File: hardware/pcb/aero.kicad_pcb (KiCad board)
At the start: 4 copper layers, 84 parts, among them CON1 USB-MICRO-B, CON2 MMCX_CONN, J1 CORTEX_DBG_CONN, J2 LiPoly_Conn, Q1 BSS138, SW1 SW_PUSH, U1 STM32L151C8, U10 BU4SU69G2, U11 BU4SU69G2, U12 NC7WZ17, U13 u-blox_max-7c/q, U14 MAX2659, U2 nRF8001, U3 2450BM14A0002, U4 ms5611, U5 BMX055, U6 AT45DB321E, U7 BQ24040DSQ, U8 TPS783, U9 TPS61041, Y1 Crystal, Y2 32.768KHz, Y3 16MHz

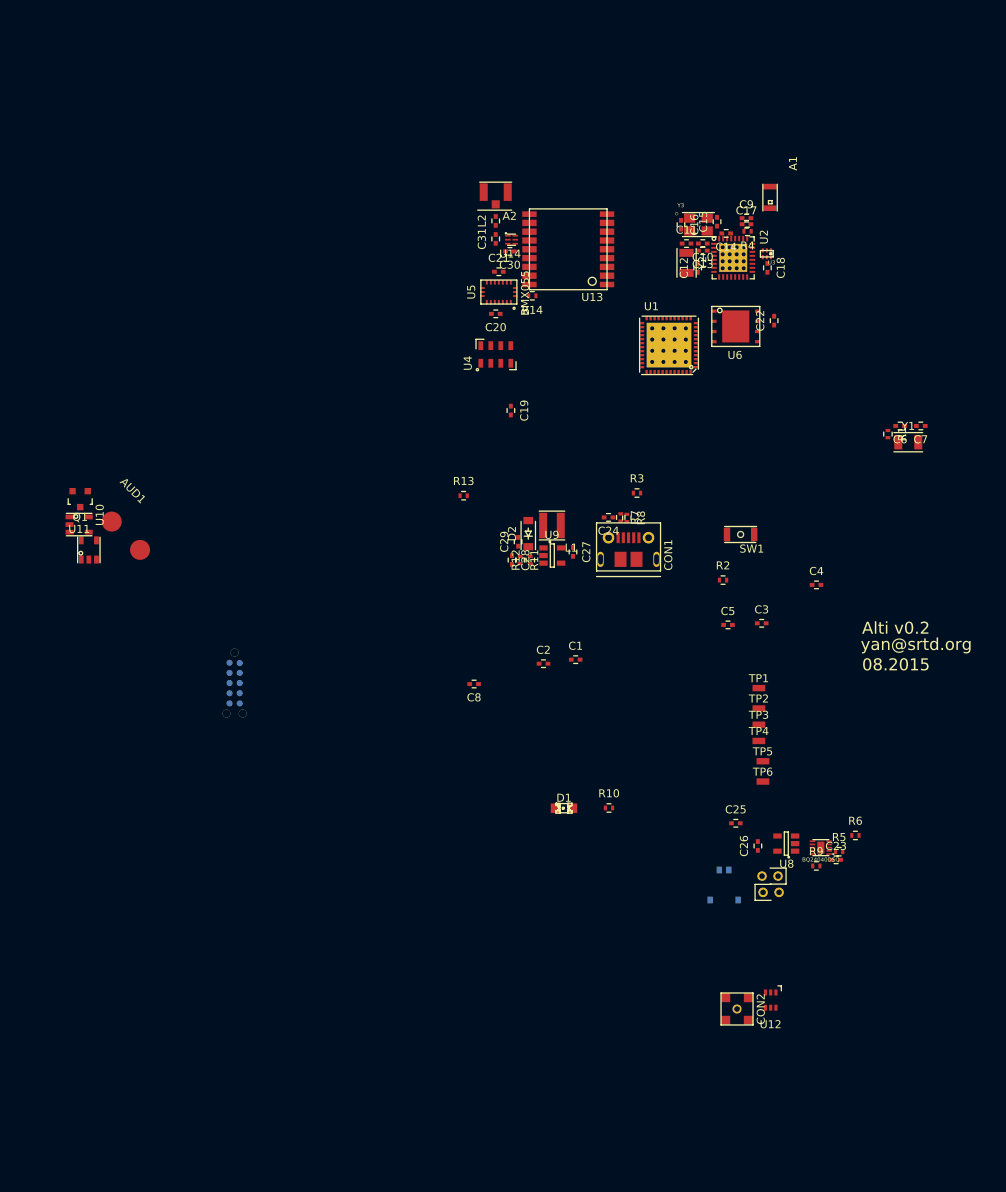
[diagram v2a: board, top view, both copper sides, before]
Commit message: ver2 is nearing completion.
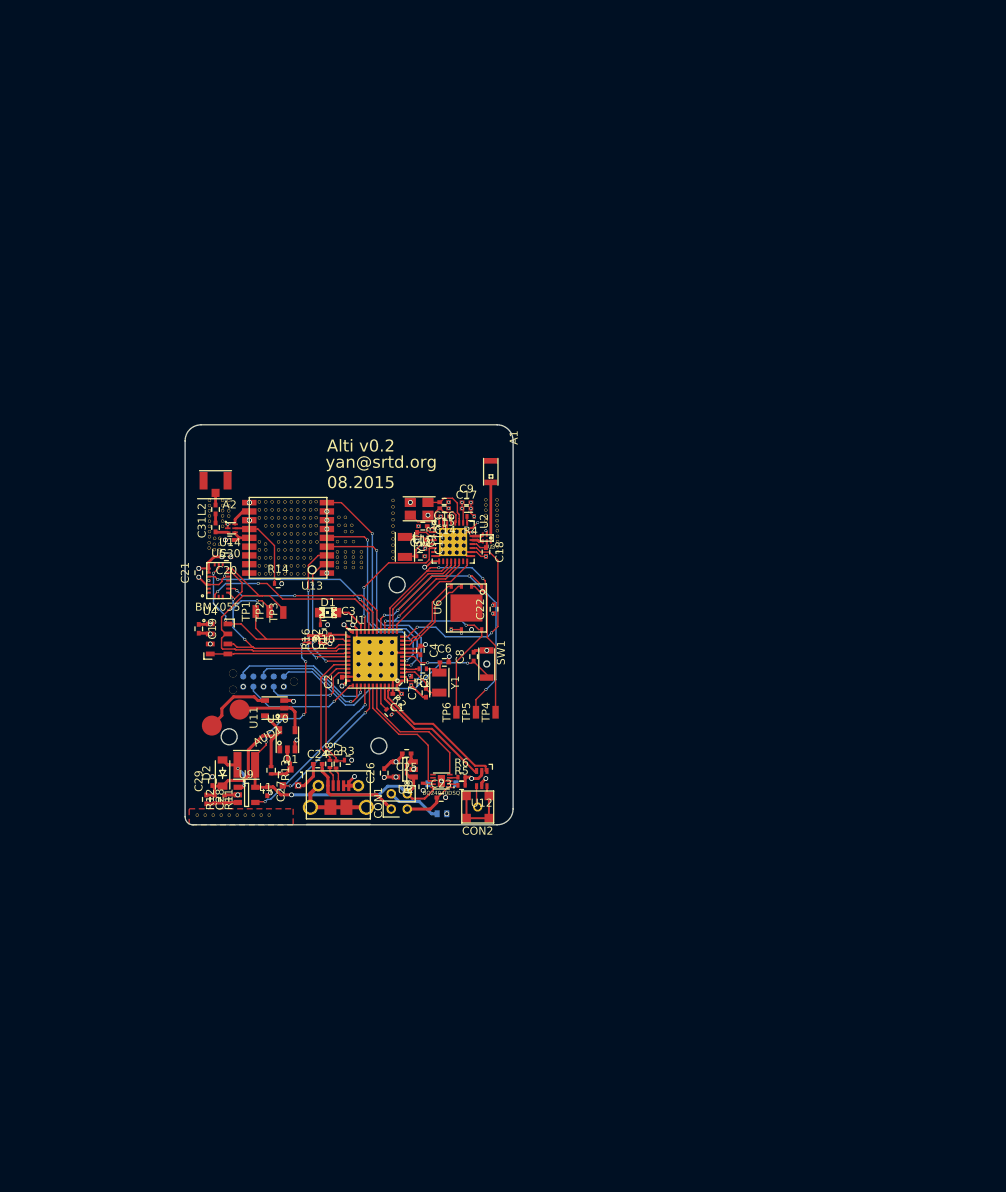
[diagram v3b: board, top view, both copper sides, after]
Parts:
- removed REF**: v, aero:Via_Stitch
- added C32: 100nF, Capacitors_SMD:C_0402, F.Cu at (143.1, 91.8)
- added R15: 10m, Resistors_SMD:R_0402, F.Cu at (140.5, 91.8)
- added R16: 10m, Resistors_SMD:R_0402, F.Cu at (141.9, 91.8)
- added REF**11101: v, aero:Via_Stitch, F.Cu at (141.4, 74.6)
- added REF**11102: v, aero:Via_Stitch, F.Cu at (141.4, 75.6)
- added REF**11103: v, aero:Via_Stitch, F.Cu at (141.4, 76.6)
- added REF**11104: v, aero:Via_Stitch, F.Cu at (141.4, 77.6)
- added REF**11105: v, aero:Via_Stitch, F.Cu at (141.4, 78.6)
- added REF**11106: v, aero:Via_Stitch, F.Cu at (141.5, 79.6)
- added REF**1111: v, aero:Via_Stitch, F.Cu at (134.3, 74.6)
- added REF**11110: v, aero:Via_Stitch, F.Cu at (134.3, 83.6)
- added REF**111101: v, aero:Via_Stitch, F.Cu at (135.5, 113.8)
- added REF**11111: v, aero:Via_Stitch, F.Cu at (126.5, 113.8)
- added REF**11111111: v, aero:Via_Stitch, F.Cu at (128.0, 80.4)
- added REF**11111111: v, aero:Via_Stitch, F.Cu at (128.0, 79.7)
- added REF**11111111: v, aero:Via_Stitch, F.Cu at (128.0, 79.0)
- added REF**11111112: v, aero:Via_Stitch, F.Cu at (129.3, 80.6)
- added REF**11111112: v, aero:Via_Stitch, F.Cu at (129.3, 79.9)
- added REF**11111112: v, aero:Via_Stitch, F.Cu at (129.3, 79.2)
- added REF**11111112: v, aero:Via_Stitch, F.Cu at (128.0, 78.3)
- added REF**11111113: v, aero:Via_Stitch, F.Cu at (128.7, 80.6)
- added REF**11111113: v, aero:Via_Stitch, F.Cu at (128.7, 79.9)
- added REF**11111113: v, aero:Via_Stitch, F.Cu at (128.7, 79.2)
- added REF**11111113: v, aero:Via_Stitch, F.Cu at (129.7, 77.7)
- added REF**11111113: v, aero:Via_Stitch, F.Cu at (128.0, 77.7)
- added REF**11111114: v, aero:Via_Stitch, F.Cu at (129.7, 77.0)
- added REF**11111114: v, aero:Via_Stitch, F.Cu at (128.0, 77.0)
- added REF**11111115: v, aero:Via_Stitch, F.Cu at (130.4, 76.4)
- added REF**11111115: v, aero:Via_Stitch, F.Cu at (129.7, 76.4)
- added REF**11111115: v, aero:Via_Stitch, F.Cu at (128.0, 76.4)
- added REF**11111116: v, aero:Via_Stitch, F.Cu at (130.4, 75.8)
- added REF**11111116: v, aero:Via_Stitch, F.Cu at (129.7, 75.7)
- added REF**11111116: v, aero:Via_Stitch, F.Cu at (128.0, 75.7)
- added REF**11111117: v, aero:Via_Stitch, F.Cu at (130.4, 75.1)
- added REF**11111117: v, aero:Via_Stitch, F.Cu at (129.7, 75.1)
- added REF**11111117: v, aero:Via_Stitch, F.Cu at (128.0, 75.1)
- added REF**11111118: v, aero:Via_Stitch, F.Cu at (130.4, 74.5)
- added REF**11111118: v, aero:Via_Stitch, F.Cu at (129.7, 74.4)
- added REF**11111118: v, aero:Via_Stitch, F.Cu at (128.0, 74.4)
- added REF**1112: v, aero:Via_Stitch, F.Cu at (134.3, 75.6)
- added REF**11121: v, aero:Via_Stitch, F.Cu at (127.5, 113.8)
- added REF**1113: v, aero:Via_Stitch, F.Cu at (134.3, 76.6)
- added REF**11131: v, aero:Via_Stitch, F.Cu at (128.5, 113.8)
- added REF**11141: v, aero:Via_Stitch, F.Cu at (129.5, 113.8)
- added REF**11151: v, aero:Via_Stitch, F.Cu at (130.5, 113.8)
- added REF**1116: v, aero:Via_Stitch, F.Cu at (134.3, 79.6)
- added REF**11161: v, aero:Via_Stitch, F.Cu at (131.5, 113.8)
- added REF**1117: v, aero:Via_Stitch, F.Cu at (134.3, 80.6)
- added REF**11171: v, aero:Via_Stitch, F.Cu at (132.5, 113.8)
- added REF**1118: v, aero:Via_Stitch, F.Cu at (134.3, 81.6)
- added REF**11181: v, aero:Via_Stitch, F.Cu at (133.5, 113.8)
- added REF**1119: v, aero:Via_Stitch, F.Cu at (134.3, 82.6)
- added REF**11191: v, aero:Via_Stitch, F.Cu at (134.5, 113.8)
- added REF**1121: v, aero:Via_Stitch, F.Cu at (135.1, 74.6)
- added REF**11210: v, aero:Via_Stitch, F.Cu at (135.1, 83.6)
- added REF**1122: v, aero:Via_Stitch, F.Cu at (135.1, 75.6)
- added REF**1123: v, aero:Via_Stitch, F.Cu at (135.1, 76.6)
- added REF**1124: v, aero:Via_Stitch, F.Cu at (135.1, 77.6)
- added REF**1126: v, aero:Via_Stitch, F.Cu at (135.1, 79.9)
- added REF**1127: v, aero:Via_Stitch, F.Cu at (135.1, 80.6)
- added REF**1128: v, aero:Via_Stitch, F.Cu at (135.1, 81.6)
- added REF**1129: v, aero:Via_Stitch, F.Cu at (135.1, 82.6)
- added REF**1131: v, aero:Via_Stitch, F.Cu at (135.9, 74.6)
- added REF**11310: v, aero:Via_Stitch, F.Cu at (135.7, 83.6)
- added REF**1132: v, aero:Via_Stitch, F.Cu at (135.9, 75.6)
- added REF**1133: v, aero:Via_Stitch, F.Cu at (135.9, 76.6)
- added REF**1134: v, aero:Via_Stitch, F.Cu at (135.9, 77.6)
- added REF**1135: v, aero:Via_Stitch, F.Cu at (135.9, 78.6)
- added REF**1138: v, aero:Via_Stitch, F.Cu at (135.7, 81.6)
- added REF**1139: v, aero:Via_Stitch, F.Cu at (135.7, 82.6)
- added REF**1141: v, aero:Via_Stitch, F.Cu at (136.7, 74.6)
- added REF**11410: v, aero:Via_Stitch, F.Cu at (136.7, 83.6)
- added REF**1142: v, aero:Via_Stitch, F.Cu at (136.7, 75.6)
- added REF**1143: v, aero:Via_Stitch, F.Cu at (136.7, 76.6)
- added REF**1144: v, aero:Via_Stitch, F.Cu at (136.7, 77.6)
- added REF**1145: v, aero:Via_Stitch, F.Cu at (136.7, 78.6)
- added REF**1146: v, aero:Via_Stitch, F.Cu at (136.7, 79.6)
- added REF**1147: v, aero:Via_Stitch, F.Cu at (136.7, 80.6)
- added REF**1148: v, aero:Via_Stitch, F.Cu at (136.7, 81.6)
- added REF**1149: v, aero:Via_Stitch, F.Cu at (136.7, 82.6)
- added REF**1151: v, aero:Via_Stitch, F.Cu at (137.5, 74.6)
- added REF**11510: v, aero:Via_Stitch, F.Cu at (137.5, 83.6)
- added REF**1152: v, aero:Via_Stitch, F.Cu at (137.5, 75.6)
- added REF**1153: v, aero:Via_Stitch, F.Cu at (137.5, 76.6)
- added REF**1154: v, aero:Via_Stitch, F.Cu at (137.5, 77.6)
- added REF**1155: v, aero:Via_Stitch, F.Cu at (137.5, 78.6)
- added REF**1156: v, aero:Via_Stitch, F.Cu at (137.5, 79.6)
- added REF**1157: v, aero:Via_Stitch, F.Cu at (137.5, 80.6)
- added REF**1158: v, aero:Via_Stitch, F.Cu at (137.5, 81.6)
- added REF**1159: v, aero:Via_Stitch, F.Cu at (137.5, 82.6)
- added REF**1161: v, aero:Via_Stitch, F.Cu at (138.3, 74.6)
- added REF**11610: v, aero:Via_Stitch, F.Cu at (138.3, 83.6)
- added REF**11611: v, aero:Via_Stitch, F.Cu at (163.3, 80.3)
- added REF**11611: v, aero:Via_Stitch, F.Cu at (164.1, 80.2)
- added REF**11611: v, aero:Via_Stitch, F.Cu at (164.0, 77.6)
- added REF**11611: v, aero:Via_Stitch, F.Cu at (162.6, 77.6)
- added REF**11612: v, aero:Via_Stitch, F.Cu at (164.1, 79.6)
- added REF**11612: v, aero:Via_Stitch, F.Cu at (164.0, 77.0)
- added REF**11612: v, aero:Via_Stitch, F.Cu at (162.6, 77.0)
- added REF**11613: v, aero:Via_Stitch, F.Cu at (164.1, 78.9)
- added REF**11613: v, aero:Via_Stitch, F.Cu at (164.0, 76.3)
- added REF**11613: v, aero:Via_Stitch, F.Cu at (162.6, 76.3)
- added REF**11614: v, aero:Via_Stitch, F.Cu at (164.0, 75.7)
- added REF**11614: v, aero:Via_Stitch, F.Cu at (162.6, 75.7)
- added REF**11615: v, aero:Via_Stitch, F.Cu at (164.0, 75.0)
- added REF**11615: v, aero:Via_Stitch, F.Cu at (162.6, 75.0)
- added REF**11616: v, aero:Via_Stitch, F.Cu at (164.1, 80.9)
- added REF**11616: v, aero:Via_Stitch, F.Cu at (164.0, 78.2)
- added REF**11616: v, aero:Via_Stitch, F.Cu at (164.0, 74.4)
- added REF**11616: v, aero:Via_Stitch, F.Cu at (162.6, 74.4)
- added REF**1162: v, aero:Via_Stitch, F.Cu at (144.2, 76.6)
- added REF**1162: v, aero:Via_Stitch, F.Cu at (138.3, 75.6)
- added REF**1163: v, aero:Via_Stitch, F.Cu at (144.2, 77.6)
- added REF**1163: v, aero:Via_Stitch, F.Cu at (138.3, 76.6)
- added REF**1164: v, aero:Via_Stitch, F.Cu at (138.3, 77.6)
- added REF**1165: v, aero:Via_Stitch, F.Cu at (138.3, 78.6)
- added REF**1166: v, aero:Via_Stitch, F.Cu at (138.3, 79.6)
- added REF**1167: v, aero:Via_Stitch, F.Cu at (138.3, 80.6)
- added REF**1168: v, aero:Via_Stitch, F.Cu at (138.3, 81.6)
- added REF**1169: v, aero:Via_Stitch, F.Cu at (138.3, 82.6)
- added REF**1171: v, aero:Via_Stitch, F.Cu at (139.1, 74.6)
- added REF**11710: v, aero:Via_Stitch, F.Cu at (139.1, 83.6)
- added REF**11711: v, aero:Via_Stitch, F.Cu at (144.1, 79.6)
- added REF**117111: v, aero:Via_Stitch, F.Cu at (144.0, 80.9)
- added REF**117112: v, aero:Via_Stitch, F.Cu at (144.0, 81.5)
- added REF**117113: v, aero:Via_Stitch, F.Cu at (144.0, 82.2)
- added REF**117114: v, aero:Via_Stitch, F.Cu at (144.0, 82.8)
- added REF**1172: v, aero:Via_Stitch, F.Cu at (145.0, 76.6)
- added REF**1172: v, aero:Via_Stitch, F.Cu at (139.1, 75.6)
- added REF**11721: v, aero:Via_Stitch, F.Cu at (145.1, 79.6)
- added REF**117211: v, aero:Via_Stitch, F.Cu at (145.0, 80.9)
- added REF**117212: v, aero:Via_Stitch, F.Cu at (145.0, 81.5)
- added REF**117213: v, aero:Via_Stitch, F.Cu at (145.0, 82.2)
- added REF**117214: v, aero:Via_Stitch, F.Cu at (145.0, 82.8)
- added REF**1173: v, aero:Via_Stitch, F.Cu at (145.0, 77.6)
- added REF**1173: v, aero:Via_Stitch, F.Cu at (139.1, 76.6)
- added REF**11731: v, aero:Via_Stitch, F.Cu at (146.1, 79.6)
- added REF**117311: v, aero:Via_Stitch, F.Cu at (146.0, 80.9)
- added REF**117311111: v, aero:Via_Stitch, F.Cu at (151.0, 74.5)
- added REF**1173111110: v, aero:Via_Stitch, F.Cu at (151.0, 81.7)
- added REF**117311112: v, aero:Via_Stitch, F.Cu at (151.0, 75.3)
- added REF**117311113: v, aero:Via_Stitch, F.Cu at (151.0, 76.1)
- added REF**117311114: v, aero:Via_Stitch, F.Cu at (151.0, 76.9)
- added REF**117311115: v, aero:Via_Stitch, F.Cu at (151.0, 77.7)
- added REF**117311116: v, aero:Via_Stitch, F.Cu at (151.0, 78.5)
- added REF**117311117: v, aero:Via_Stitch, F.Cu at (151.0, 79.3)
- added REF**117311118: v, aero:Via_Stitch, F.Cu at (151.0, 80.1)
- added REF**117311119: v, aero:Via_Stitch, F.Cu at (151.0, 80.9)
- added REF**117312: v, aero:Via_Stitch, F.Cu at (146.0, 81.5)
- added REF**117313: v, aero:Via_Stitch, F.Cu at (146.0, 82.2)
- added REF**117314: v, aero:Via_Stitch, F.Cu at (146.0, 82.8)
- added REF**1174: v, aero:Via_Stitch, F.Cu at (145.0, 78.3)
- added REF**1174: v, aero:Via_Stitch, F.Cu at (139.1, 77.6)
- added REF**117411: v, aero:Via_Stitch, F.Cu at (147.0, 80.9)
- added REF**117412: v, aero:Via_Stitch, F.Cu at (147.0, 81.5)
- added REF**117413: v, aero:Via_Stitch, F.Cu at (147.0, 82.2)
- added REF**117414: v, aero:Via_Stitch, F.Cu at (147.0, 82.8)
- added REF**1175: v, aero:Via_Stitch, F.Cu at (139.1, 78.6)
- added REF**1176: v, aero:Via_Stitch, F.Cu at (139.1, 79.6)
- added REF**1177: v, aero:Via_Stitch, F.Cu at (139.1, 80.6)
- added REF**1178: v, aero:Via_Stitch, F.Cu at (139.1, 81.6)
- added REF**1179: v, aero:Via_Stitch, F.Cu at (139.1, 82.6)
- added REF**1181: v, aero:Via_Stitch, F.Cu at (139.9, 74.6)
- added REF**11810: v, aero:Via_Stitch, F.Cu at (139.9, 83.6)
- added REF**1182: v, aero:Via_Stitch, F.Cu at (139.9, 75.6)
- added REF**1183: v, aero:Via_Stitch, F.Cu at (145.8, 77.6)
- added REF**1183: v, aero:Via_Stitch, F.Cu at (139.9, 76.6)
- added REF**1184: v, aero:Via_Stitch, F.Cu at (145.8, 78.3)
- added REF**1184: v, aero:Via_Stitch, F.Cu at (139.9, 77.6)
- added REF**1185: v, aero:Via_Stitch, F.Cu at (139.9, 78.6)
- added REF**1186: v, aero:Via_Stitch, F.Cu at (139.9, 79.6)
- added REF**1187: v, aero:Via_Stitch, F.Cu at (139.9, 80.6)
- added REF**1188: v, aero:Via_Stitch, F.Cu at (139.9, 81.6)
- added REF**1189: v, aero:Via_Stitch, F.Cu at (139.9, 82.6)
- added REF**1191: v, aero:Via_Stitch, F.Cu at (140.7, 74.6)
- added REF**1192: v, aero:Via_Stitch, F.Cu at (140.7, 75.6)
- added REF**1193: v, aero:Via_Stitch, F.Cu at (140.7, 76.6)
- added REF**1194: v, aero:Via_Stitch, F.Cu at (140.7, 77.6)
- added REF**1195: v, aero:Via_Stitch, F.Cu at (140.7, 78.6)
- added REF**1196: v, aero:Via_Stitch, F.Cu at (140.7, 79.6)
- added REF**1197: v, aero:Via_Stitch, F.Cu at (140.7, 80.6)
- added REF**1198: v, aero:Via_Stitch, F.Cu at (140.7, 81.6)
- moved C7 70.3 mm to (155.1, 98.5), turned to 90 degrees
- moved Y1 65.9 mm to (156.8, 97.2), turned to 270 degrees
- moved R1 65.1 mm to (154.7, 95.5), turned to 180 degrees
- moved C6 64.2 mm to (157.4, 94.7), turned to 0 degrees
- moved TP1 63.6 mm to (133.8, 88.3), turned to 180 degrees
- moved TP2 62.4 mm to (135.5, 88.3), turned to 180 degrees
- moved TP3 61.1 mm to (137.3, 88.5), turned to 180 degrees
- moved U1 53.7 mm to (148.8, 94.2)
- moved C21 53.1 mm to (126.7, 83.5), turned to 90 degrees
- moved C3 51.7 mm to (145.4, 90.0)
- moved C13 50.5 mm to (154.0, 79.0), turned to 270 degrees
- moved C30 50.3 mm to (130.6, 79.4)
- moved U5 50.3 mm to (129.2, 84.5), turned to 180 degrees
- moved C31 50.3 mm to (128.8, 77.8)
- moved L2 50.3 mm to (128.8, 75.6)
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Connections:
- CON1 pad 10: (no net) -> GND
- CON1 pad 11: (no net) -> GND
- U1 pad 25: /ms5611/EN -> BATT_SENSE
- U1 pad 29: Net-(U1-Pad29) -> MS5611_EN
- U1 pad 30: ~PG -> GPS_RX
- U1 pad 31: ~CHG -> GPS_TX
- U1 pad 42: /GPS/RxD -> ~CHG
- U1 pad 43: /GPS/TxD -> ~PG
- U1 pad 49: (no net) -> GND
- U13 pad 2: /GPS/TxD -> GPS_TX
- U13 pad 3: /GPS/RxD -> GPS_RX
- U2 pad 33: (no net) -> GND
- U4 pad 4: /ms5611/EN -> MS5611_EN
- U4 pad 5: /ms5611/EN -> MS5611_EN
- U7 pad 11: (no net) -> GND
- Y3 pad 3: (no net) -> GND
- Y3 pad 4: (no net) -> GND
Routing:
- net GND: track 0.00 -> 80.7 mm, vias 0 -> 53
- net Vbatt: track 0.00 -> 54.5 mm, vias 0 -> 5
- net /at45db321e/MOSI: track 0.00 -> 46.5 mm, vias 0 -> 4
- net /at45db321e/SCK: track 0.00 -> 40.5 mm, vias 0 -> 2
- net /at45db321e/MISO: track 0.00 -> 38.1 mm, vias 0 -> 3
- net /bmx055/MOSI: track 0.00 -> 36.3 mm
- net ~NRST: track 0.00 -> 36.2 mm, vias 0 -> 2
- net /bmx055/MISO: track 0.00 -> 34.2 mm, vias 0 -> 3
- net /GPS/RESET: track 0.00 -> 29.5 mm, vias 0 -> 2
- net /GPS/TIMEPULSE: track 0.00 -> 29.2 mm, vias 0 -> 2
- net /bmx055/SCK: track 0.00 -> 28.4 mm, vias 0 -> 2
- net +3V: track 0.00 -> 25.9 mm, vias 0 -> 26
- net /nRF8001/~RESET: track 0.00 -> 25.6 mm, vias 0 -> 2
- net /GPS/EXT_INT: track 0.00 -> 25.5 mm, vias 0 -> 2
- net /bmx055/GYRO_SEL: track 0.00 -> 24.8 mm, vias 0 -> 2
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- added copper zone on In2.Cu, net +3V
- added copper zone on F.Cu, net GND
- added copper zone on In1.Cu, net GND
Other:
- board outline added: 41 x 50 mm
- net class Default: clearance 0.2 -> 0.1524
- rule trace_clearance: 0.2 -> 0.1524
